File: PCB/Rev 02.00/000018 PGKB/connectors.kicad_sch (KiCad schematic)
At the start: 3 parts, among them J2 BM04B-SRSS-TB

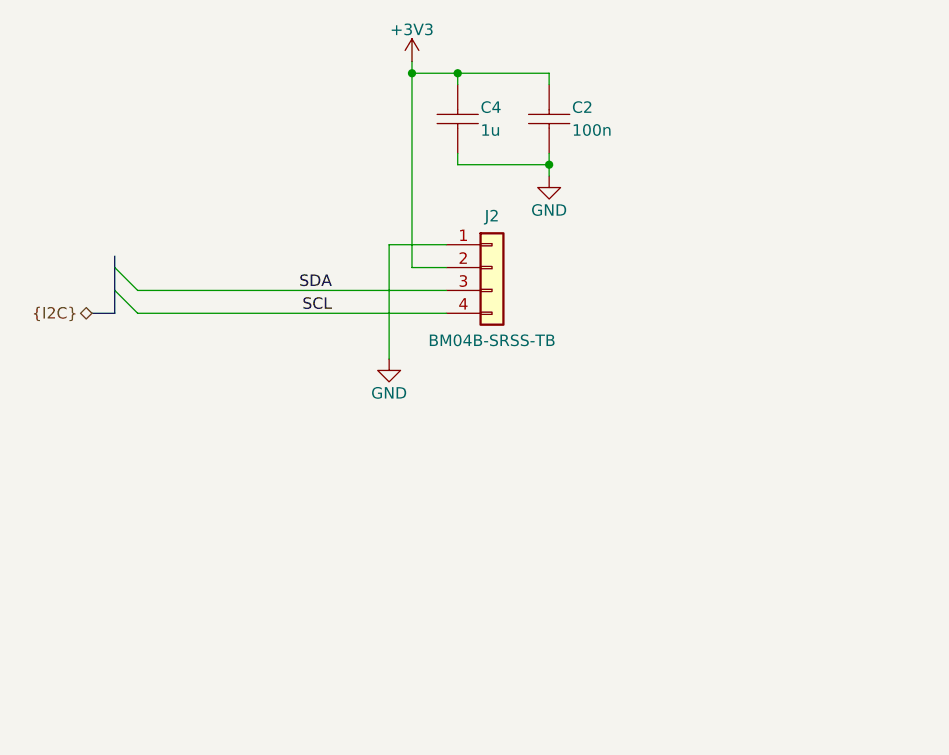
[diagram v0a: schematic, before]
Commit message: Schematic
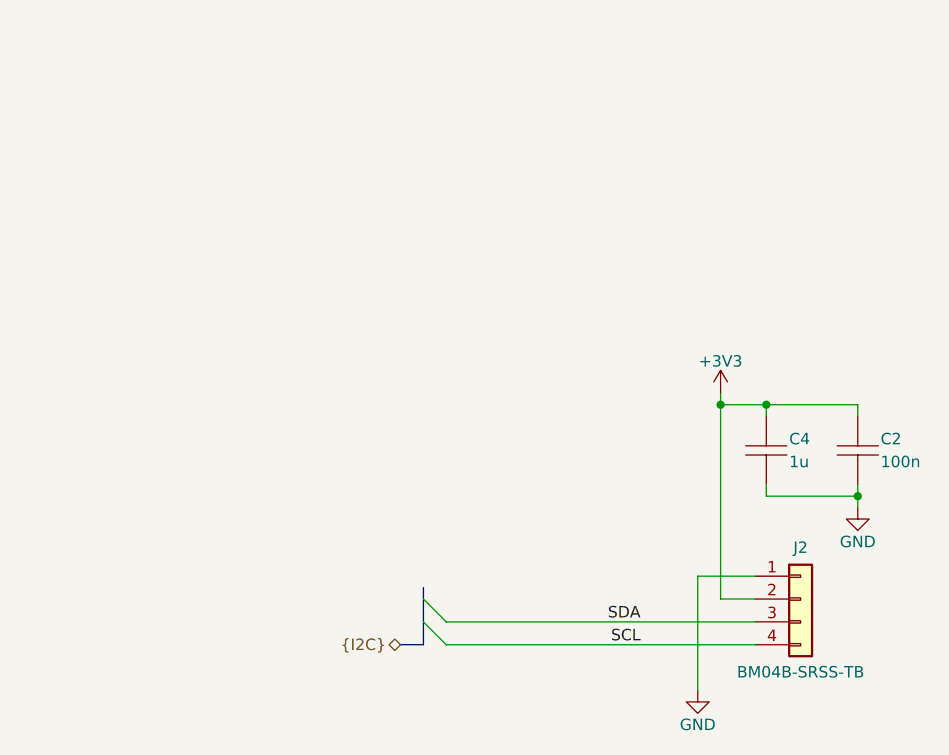
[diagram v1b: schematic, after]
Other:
- company: (none) -> Kallio Designs Oy
- title: (none) -> Programmable Keyboard
- moved on the sheet: C2, C4, J2

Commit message: updates
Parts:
- J2: footprint KD_Connector_Rectangular:JST_SH_BM04B-SRSS-TB_1x04-1MP_P1.00mm_Vertical -> KD_Connector_Rectangular:JST_PH_S4B-PH-SM4-TB_1x04-1MP_P2.00mm_Horizontal; symbol KD_Connector_Rectangular:JST_SH_1X04_BM04B-SRSS-TB -> KD_Connector_Rectangular:JST_PH_1X04_S4B-PH-SM4-TB; MFG_PartNo BM04B-SRSS-TB -> S4B-PH-SM4-TB; Price 1.5 -> 0.7; Supplier_PartNo 455-BM04B-SRSS-TBCT-ND -> 455-S4B-PH-SM4-TBCT-ND
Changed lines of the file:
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@@
         )
         (path "/e63e39d7-6ac0-4ffd-8aa3-1841a4541b55/2eb44e1a-4042-4ea6-aca2-4836a6ec84e9/4ce60c68-8f85-4df7-a465-152e58489d9e"
-          (reference "#GND022") (unit 1)
+          (reference "#GND012") (unit 1)
         )
       )
@@
         )
         (path "/e63e39d7-6ac0-4ffd-8aa3-1841a4541b55/2eb44e1a-4042-4ea6-aca2-4836a6ec84e9/4ce60c68-8f85-4df7-a465-152e58489d9e"
-          (reference "#GND021") (unit 1)
+          (reference "#GND011") (unit 1)
         )
       )
@@
         )
         (path "/e63e39d7-6ac0-4ffd-8aa3-1841a4541b55/2eb44e1a-4042-4ea6-aca2-4836a6ec84e9/4ce60c68-8f85-4df7-a465-152e58489d9e"
-          (reference "C23") (unit 1)
-        )
-      )
-    )
-  )
-  (symbol (lib_id "KD_Connector_Rectangular:JST_SH_1X04_BM04B-SRSS-TB") (at 156.21 100.33 0) (unit 1)
+          (reference "C21") (unit 1)
+        )
+      )
+    )
+  )
+  (symbol (lib_id "KD_Connector_Rectangular:JST_PH_1X04_S4B-PH-SM4-TB") (at 156.21 100.33 0) (unit 1)
     (in_bom yes) (on_board yes) (dnp no)
     (property "Reference" "J2" (at 161.29 97.155 0) (do_not_autoplace)
@@
       (effects (font (size 1.27 1.27)))
     )
-    (property "Footprint" "KD_Connector_Rectangular:JST_SH_BM04B-SRSS-TB_1x04-1MP_P1.00mm_Vertical" (at 143.51 86.36 0)
-      (effects (font (size 1.27 1.27)) (justify left) hide)
-    )
-    (property "Datasheet" "https://www.jst-mfg.com/product/pdf/eng/eSH.pdf" (at 143.51 88.9 0)
+    (property "Footprint" "KD_Connector_Rectangular:JST_PH_S4B-PH-SM4-TB_1x04-1MP_P2.00mm_Horizontal" (at 143.51 86.36 0)
+      (effects (font (size 1.27 1.27)) (justify left) hide)
+    )
+    (property "Datasheet" "https://www.jst-mfg.com/product/pdf/eng/ePH.pdf" (at 143.51 88.9 0)
       (effects (font (size 1.27 1.27)) (justify left) hide)
     )
@@
       (effects (font (size 1.27 1.27)) (justify left) hide)
     )
-    (property "MFG_PartNo" "BM04B-SRSS-TB" (at 143.51 73.66 0)
+    (property "MFG_PartNo" "S4B-PH-SM4-TB" (at 143.51 73.66 0)
       (effects (font (size 1.27 1.27)) (justify left) hide)
     )
@@
       (effects (font (size 1.27 1.27)) (justify left) hide)
     )
-    (property "Supplier_PartNo" "455-BM04B-SRSS-TBCT-ND" (at 143.51 78.74 0)
+    (property "Supplier_PartNo" "455-S4B-PH-SM4-TBCT-ND" (at 143.51 78.74 0)
       (effects (font (size 1.27 1.27)) (justify left) hide)
     )
@@
       (effects (font (size 1.27 1.27)) (justify left) hide)
     )
-    (property "Price" "1.5" (at 143.51 83.82 0)
+    (property "Price" "0.7" (at 143.51 83.82 0)
       (effects (font (size 1.27 1.27)) (justify left) hide)
     )
@@
         )
         (path "/e63e39d7-6ac0-4ffd-8aa3-1841a4541b55/2eb44e1a-4042-4ea6-aca2-4836a6ec84e9/4ce60c68-8f85-4df7-a465-152e58489d9e"
-          (reference "#+3V010") (unit 1)
+          (reference "#+3V03") (unit 1)
         )
       )
@@
         )
         (path "/e63e39d7-6ac0-4ffd-8aa3-1841a4541b55/2eb44e1a-4042-4ea6-aca2-4836a6ec84e9/4ce60c68-8f85-4df7-a465-152e58489d9e"
-          (reference "C24") (unit 1)
-        )
-      )
+          (reference "C22") (unit 1)
+        )
+      )
